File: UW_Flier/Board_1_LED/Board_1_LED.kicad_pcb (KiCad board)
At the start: 2 copper layers, 9.2 x 10.5 mm, 11 parts, among them J1 RESET, J2 SWDIO, J3 SWDCLK, J4 GND, J5 VDD, J6 LED_DRAIN, Q1 CSD13385F5, U1 EYSHSNZWZ_module_stub

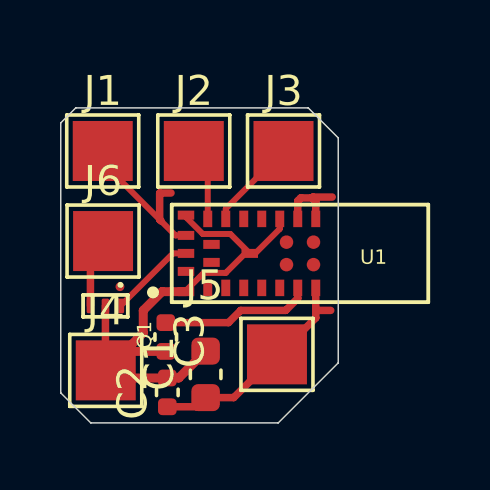
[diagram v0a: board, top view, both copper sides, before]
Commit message: updated PCB
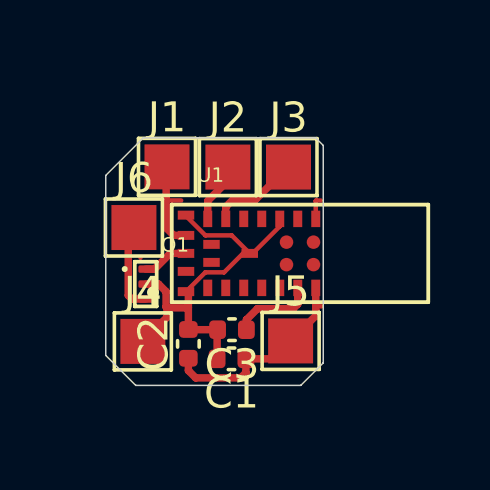
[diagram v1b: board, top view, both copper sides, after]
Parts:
- C1: footprint Capacitor_SMD:C_0603_1608Metric -> Capacitor_SMD:C_0402_1005Metric
- J1, J2, J3, J4, J5, J6: footprint TestPoint:TestPoint_Pad_2.0x2.0mm -> CSD13385F5:TestPoint_Pad_1.5x1.5mm_2
- moved C3 2.22 mm to (106.7, 76.9), turned to 180 degrees
- moved J1 2.21 mm to (104.5, 71.5)
- moved C2 1.76 mm to (105.3, 77.4)
- moved J4 1.57 mm to (103.7, 77.3)
- moved Q1 1.53 mm to (103.8, 75.4), turned to 0 degrees
- moved J2 1.26 mm to (106.6, 71.5)
- moved J6 1.12 mm to (103.4, 73.5)
- moved C1 1.01 mm to (106.7, 77.9), turned to 180 degrees
- moved J5 0.64 mm to (108.7, 77.3)
- moved J3 0.56 mm to (108.6, 71.5)
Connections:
- Q1 pad 2: Net-(J6-Pin_1) -> Net-(J4-Pin_1)
- Q1 pad 3: Net-(J4-Pin_1) -> Net-(J6-Pin_1)
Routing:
- net Net-(J4-Pin_1): track 20.2 -> 13.7 mm
- net unconnected-(U1-OUT_MOD-Pad12): track 2.35 -> 0.00 mm
- net Net-(U1-DEC4): track 5.08 -> 2.80 mm
- net Net-(J1-Pin_1): track 5.54 -> 3.31 mm
- net Net-(Q1-G): track 2.91 -> 1.56 mm
- net unconnected-(U1-OUT_ANT-Pad11): track 0.00 -> 0.78 mm
- net Net-(J5-Pin_1): track 7.67 -> 7.02 mm
- net Net-(J6-Pin_1): track 2.45 -> 2.97 mm
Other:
- board size 9.2 x 10.5 mm -> 7.2 x 8.2 mm
- board text removed: "${REFERENCE}"
